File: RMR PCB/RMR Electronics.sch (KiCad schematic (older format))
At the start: 15 parts, among them J1 RasPi Power, J2 Arduino Power, J3 Left Servo, J4 Right Servo, J5 Mast Servo, U1 LD1117S18TR_SOT223, U2 LD1117S18TR_SOT223

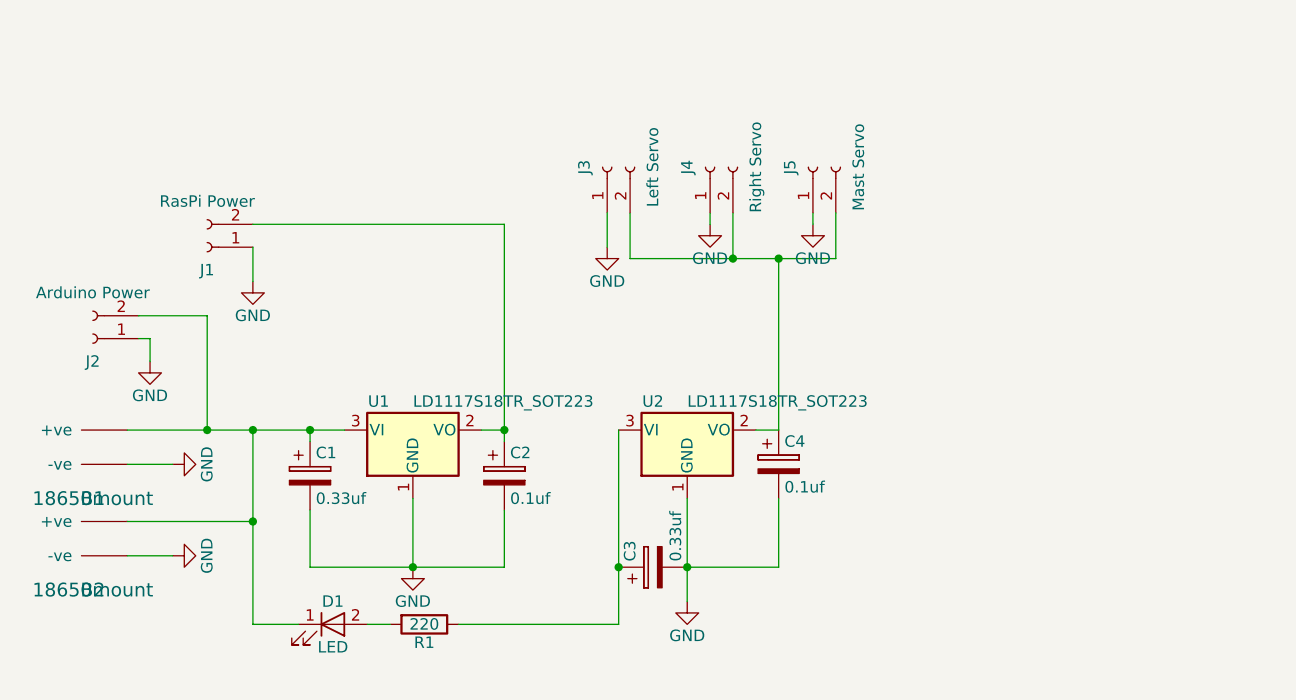
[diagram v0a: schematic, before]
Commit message: Finished layout
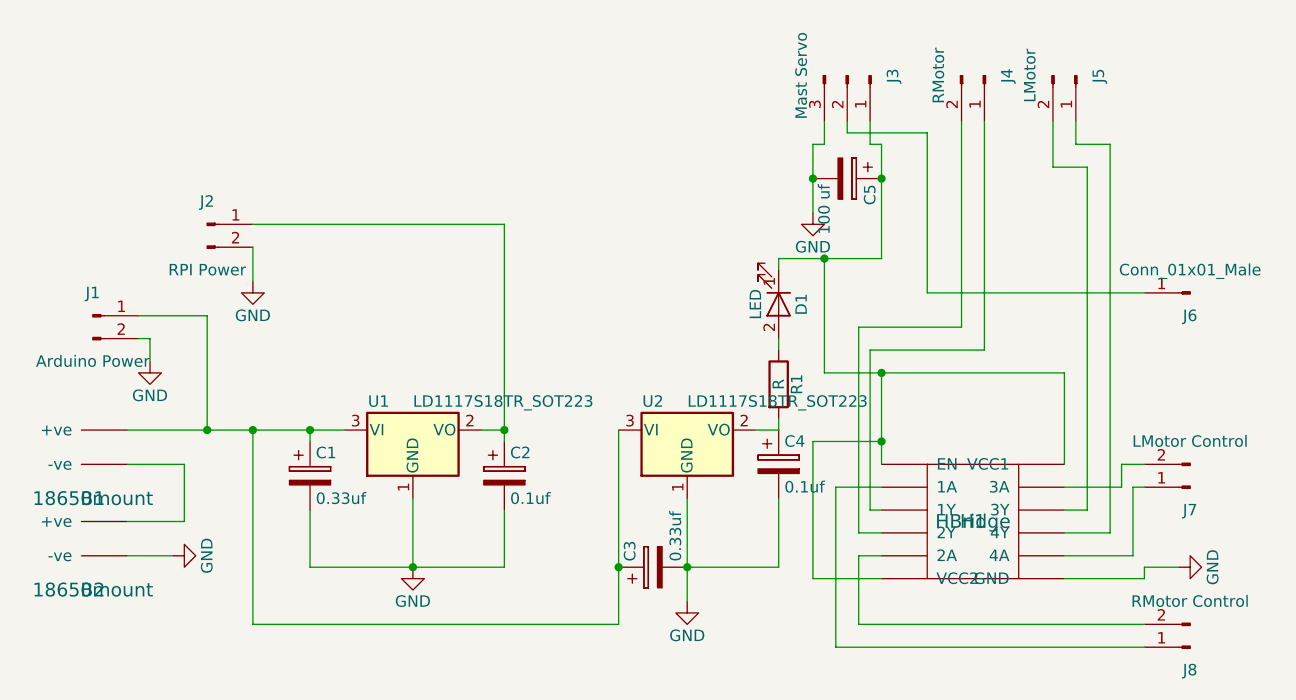
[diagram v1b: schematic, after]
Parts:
- removed J1: RasPi Power, symbol Conn_01x02_Female
- removed J2: Arduino Power, symbol Conn_01x02_Female
- removed J3: Left Servo, symbol Conn_01x02_Female
- removed J4: Right Servo, symbol Conn_01x02_Female
- removed J5: Mast Servo, symbol Conn_01x02_Female
- added C5: 100 uf, symbol CP
- added H1: HBridge, symbol HBridge
- added J1: Arduino Power, symbol Conn_01x02_Male
- added J2: RPI Power, symbol Conn_01x02_Male
- added J3: Mast Servo, symbol Conn_01x03_Male
- added J4: RMotor, symbol Conn_01x02_Male
- added J5: LMotor, symbol Conn_01x02_Male
- added J6: Conn_01x01_Male, symbol Conn_01x01_Male
- added J7: LMotor Control, symbol Conn_01x02_Male
- added J8: RMotor Control, symbol Conn_01x02_Male
- R1: value 220 -> R
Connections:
- net GND: now also C5.2, H1.~ (VCC2), J1.2 (Pin_2), J2.2 (Pin_2), J3.3 (Pin_3); no longer B1.~ (-ve)
- net at C2.1, U1.2 (VO): now also J2.1 (Pin_1)
- net at C4.1, U2.2 (VO): now also R1.2
- net at C3.1, U2.3 (VI): now also B1.~ (-ve), C1.1, U1.3 (VI), J1.1 (Pin_1); no longer R1.1
- net at D1.2 (A): now also R1.1; no longer R1.2
- new net: B1.~ (-ve), B2.~ (-ve)
- new net: C5.1, D1.1 (K), H1.~ (VCC2), J3.1 (Pin_1)
- new net: J3.2 (Pin_2), J6.1 (Pin_1)
- new net: H1.~ (VCC2), J8.1 (Pin_1)
- new net: H1.~ (VCC2), J8.2 (Pin_2)
- new net: H1.~ (VCC2), J7.1 (Pin_1)
- new net: H1.~ (VCC2), J7.2 (Pin_2)
- new net: H1.~ (VCC2), J4.1 (Pin_1)
- new net: H1.~ (VCC2), J4.2 (Pin_2)
- new net: H1.~ (VCC2), J5.1 (Pin_1)
- new net: H1.~ (VCC2), J5.2 (Pin_2)
